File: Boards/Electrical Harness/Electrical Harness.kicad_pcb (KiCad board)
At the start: 4 copper layers, 48.5 x 38.1 mm, 4 parts, among them J1 10-18-1041, J2 39-28-8080, J3 39-28-8080, J4 10-18-1041

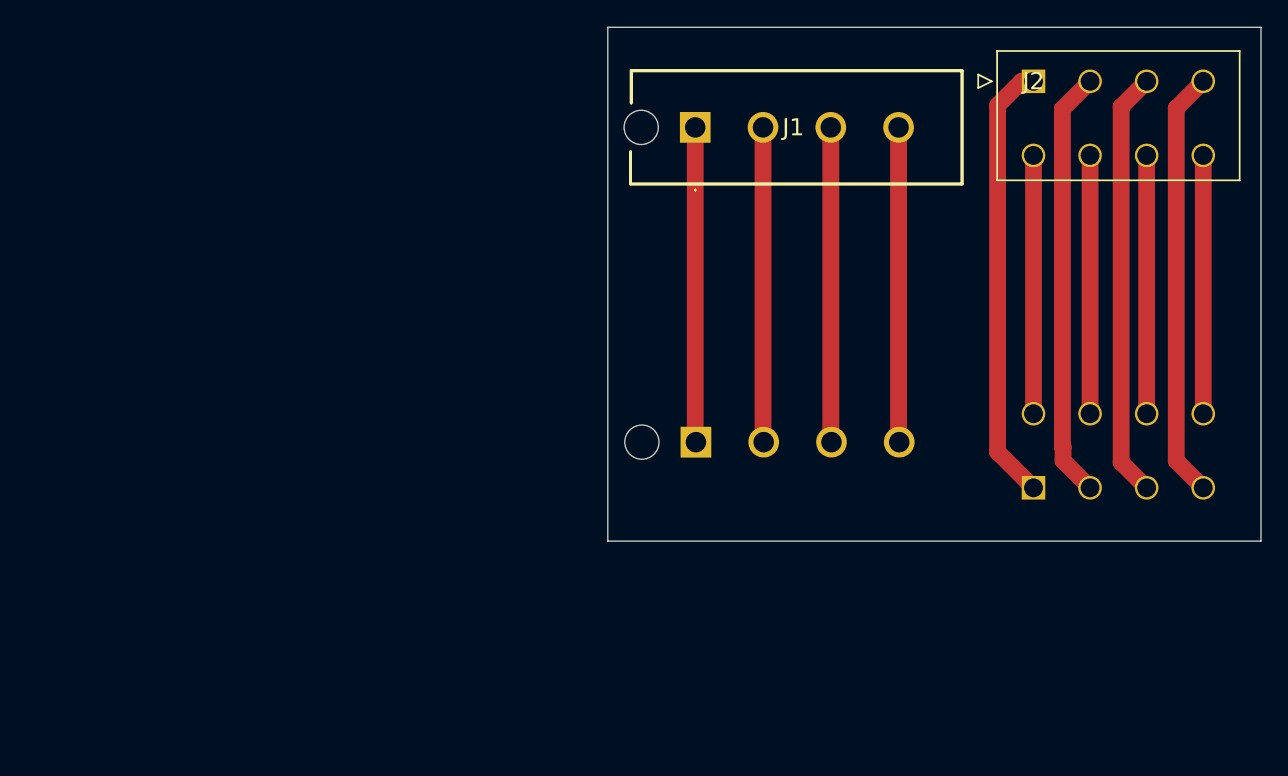
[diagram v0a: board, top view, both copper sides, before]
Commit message: PCB CALHA
PCB CALHA
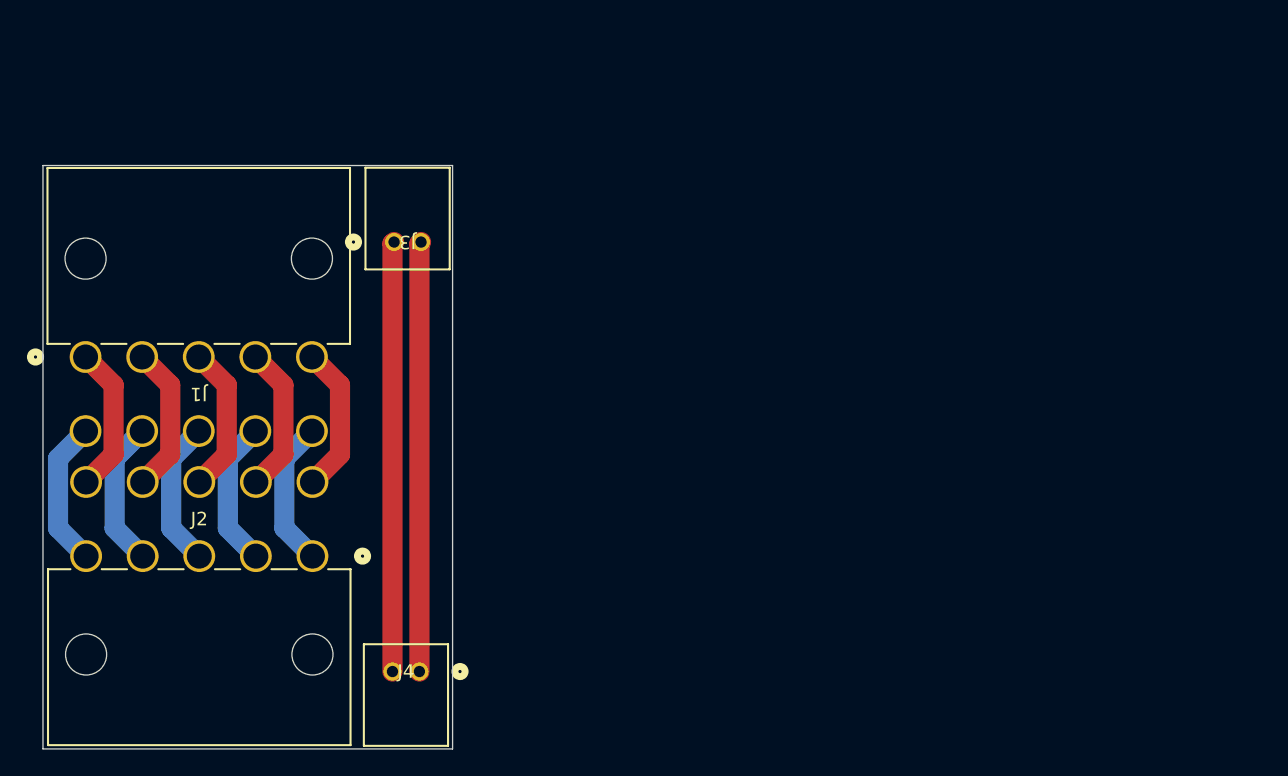
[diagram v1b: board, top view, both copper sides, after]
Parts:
- J1: value 10-18-1041 -> 39300100; footprint 10-18-1041:10181041 -> CONN_5569-10A_MOL:CONN_5569-10A_MOL
- J2: value 39-28-8080 -> 39300100; footprint 39-28-8080:39-28-8080 -> CONN_5569-10A_MOL:CONN_5569-10A_MOL
- J3: value 39-28-8080 -> 532540270; footprint 39-28-8080:39-28-8080 -> CONN02_532540270_MOL:CONN02_532540270_MOL; moved to F.Cu
- J4: value 10-18-1041 -> 532540270; footprint 10-18-1041:10181041 -> CONN02_532540270_MOL:CONN02_532540270_MOL; moved to F.Cu
- moved J2 64.1 mm to (148.6, 75.4)
- moved J3 50.8 mm to (154.7, 52.1), turned to 180 degrees
- moved J1 48.4 mm to (131.8, 60.6)
- moved J4 26.7 mm to (156.5, 84.0), turned to 0 degrees
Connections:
- J2 pad 1: Net-(J2-Pad1) -> Net-(J1-Pad10)
- J2 pad 2: Net-(J2-Pad2) -> Net-(J1-Pad9)
- J2 pad 3: Net-(J2-Pad3) -> Net-(J1-Pad8)
- J2 pad 4: Net-(J2-Pad4) -> Net-(J1-Pad7)
- J2 pad 5: Net-(J2-Pad5) -> Net-(J1-Pad6)
- J2 pad 6: Net-(J2-Pad6) -> Net-(J1-Pad5)
- J2 pad 7: Net-(J2-Pad7) -> Net-(J1-Pad4)
- J2 pad 8: Net-(J2-Pad8) -> Net-(J1-Pad3)
- J3 pad 1: Net-(J2-Pad1) -> Net-(J3-Pad1)
- J3 pad 2: Net-(J2-Pad2) -> Net-(J3-Pad2)
- J4 pad 1: Net-(J1-Pad1) -> Net-(J3-Pad2)
- J4 pad 2: Net-(J1-Pad2) -> Net-(J3-Pad1)
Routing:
- net Net-(J2-Pad1): track 32.9 -> 0.00 mm
- net Net-(J3-Pad2): track 0.00 -> 31.9 mm
- net Net-(J3-Pad1): track 0.00 -> 31.9 mm
- net Net-(J2-Pad2): track 31.9 -> 0.00 mm
- net Net-(J2-Pad4): track 31.8 -> 0.00 mm
- net Net-(J2-Pad3): track 31.7 -> 0.00 mm
- net Net-(J2-Pad8): track 19.2 -> 0.00 mm
- net Net-(J2-Pad7): track 19.2 -> 0.00 mm
- net Net-(J2-Pad6): track 19.2 -> 0.00 mm
- net Net-(J2-Pad5): track 19.2 -> 0.00 mm
- net Net-(J1-Pad4): track 23.4 -> 11.0 mm
- net Net-(J1-Pad2): track 23.4 -> 11.0 mm
- net Net-(J1-Pad3): track 23.4 -> 11.0 mm
- net Net-(J1-Pad1): track 23.4 -> 11.0 mm
- net Net-(J1-Pad6): track 0.00 -> 11.1 mm
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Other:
- board size 48.5 x 38.1 mm -> 30.4 x 43.3 mm
